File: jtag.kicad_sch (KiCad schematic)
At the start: 49 parts, among them J3 USB_C_Receptacle, J4 Conn_01x02_Male, J5 3220-10-0100-00, U2 FT2232HL-REEL, U3 74LVC1G125, U4 74LVC1G125, U5 74LVC1G125, U6 74LVC1G125, U7 74LVC1G125, Y2 12MHz

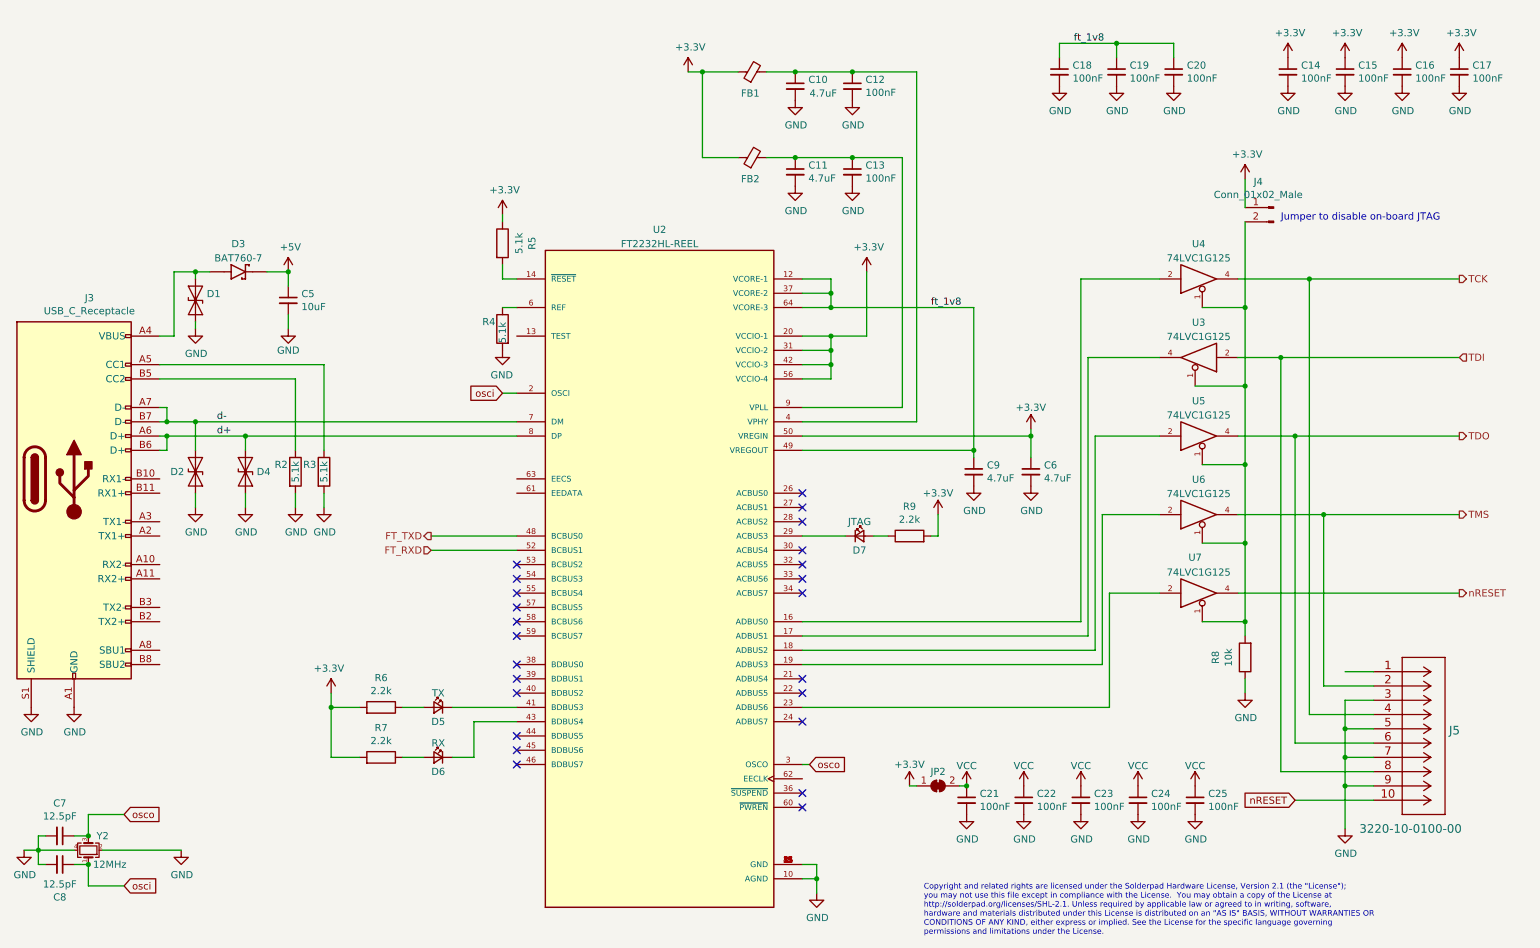
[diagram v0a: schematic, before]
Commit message: Power and Level Shifter updates
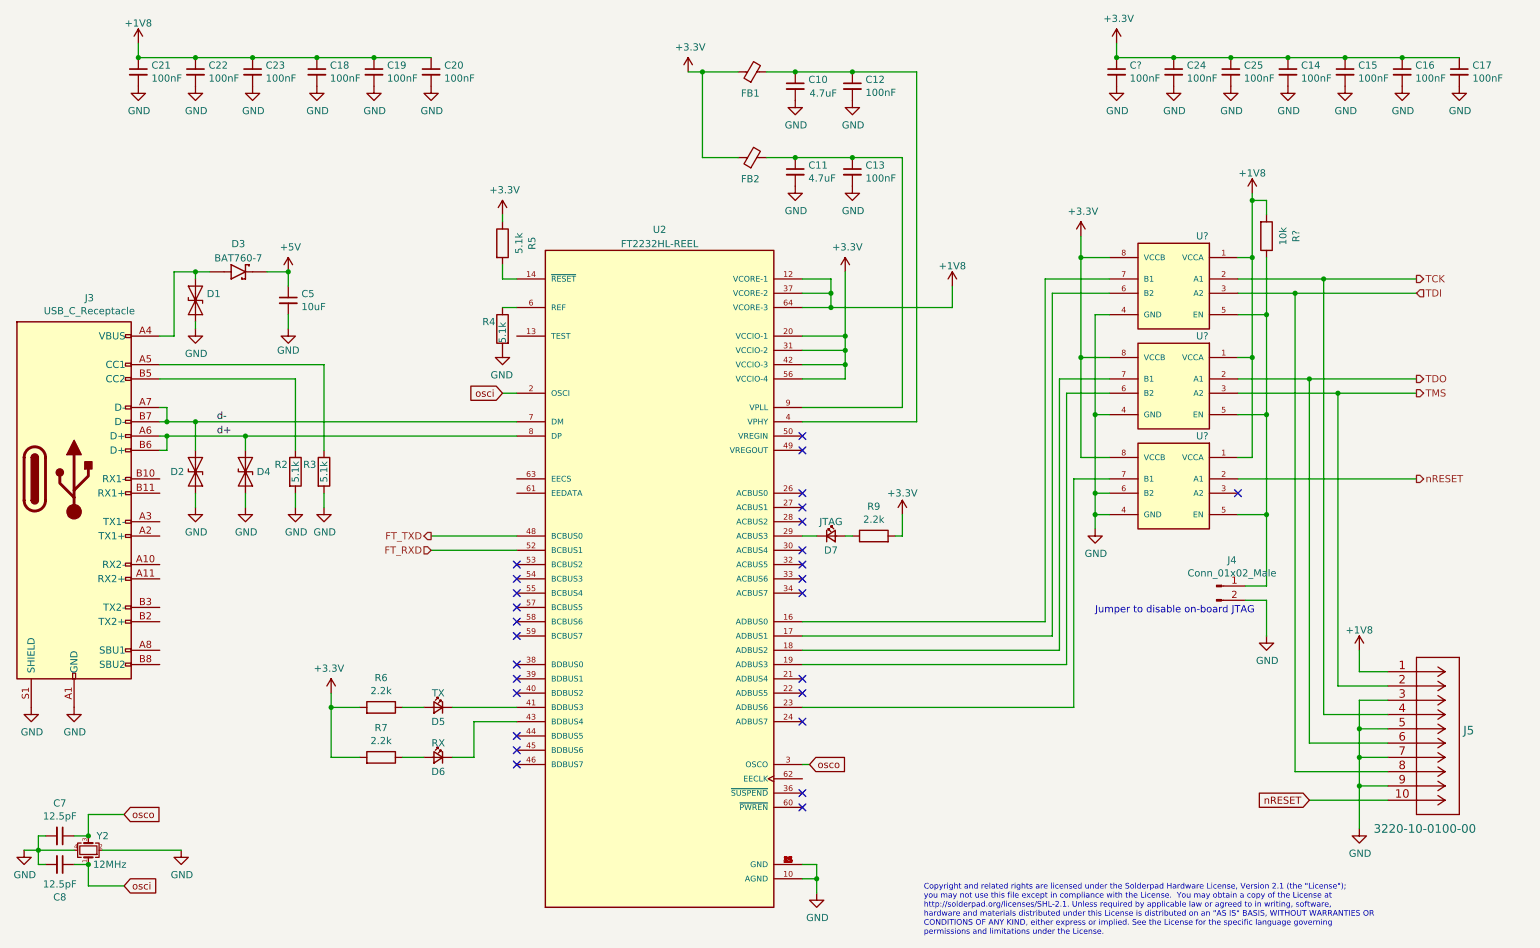
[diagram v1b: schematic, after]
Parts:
- removed C6, C9: 4.7uF, Capacitor_SMD:C_0603_1608Metric_Pad1.08x0.95mm_HandSolder, symbol Device:C_Small
- removed JP2: SolderJumper_2_Bridged, Jumper:SolderJumper-2_P1.3mm_Bridged_RoundedPad1.0x1.5mm, symbol Jumper:SolderJumper_2_Bridged
- removed R8: 10k, Resistor_SMD:R_0603_1608Metric_Pad0.98x0.95mm_HandSolder, symbol Device:R
- removed U3, U4, U5, U6, U7: 74LVC1G125, Package_TO_SOT_SMD:SOT-353_SC-70-5, symbol 74xGxx:74LVC1G125
- added C?: 100nF, Capacitor_SMD:C_0603_1608Metric_Pad1.08x0.95mm_HandSolder, symbol Device:C_Small
- added R?: 10k, Resistor_SMD:R_0603_1608Metric_Pad0.98x0.95mm_HandSolder, symbol Device:R
- added U? (x3): PI4ULS3V302XVEX, PSON40P160X120X55-8N, symbol PI4ULS3V302XVEX:PI4ULS3V302XVEX
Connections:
- net +3V3: now also C24.1, C25.1, C?.1, U?.8 (VCCB), U?.8 (VCCB), U?.8 (VCCB); no longer J4.1 (Pin_1), U2.50 (VREGIN)
- net GND: now also J4.2 (Pin_2), C?.2, U?.4 (GND), U?.4 (GND), U?.4 (GND), U?.6 (B2)
- net TCK: now also U?.2 (A1)
- net TDI: now also U?.3 (A2)
- net TDO: now also U?.2 (A1)
- net TMS: now also U?.3 (A2)
- net nRESET: now also U?.2 (A1)
- net at U2.19 (ADBUS3): now also U?.6 (B2)
- net at U2.23 (ADBUS6): now also U?.7 (B1)
- net at U2.18 (ADBUS2): now also U?.7 (B1)
- net +1V8: now reaches J5.1
- net +1V8: now also C18.1, C19.1, C20.1, C21.1, C22.1, C23.1, U2.12 (VCORE-1), U2.37 (VCORE-2), U2.64 (VCORE-3), R?.2, U?.1 (VCCA), U?.1 (VCCA), U?.1 (VCCA)
- net at U2.16 (ADBUS0): now also U?.7 (B1)
- net at U2.17 (ADBUS1): now also U?.6 (B2)
- removed net VCC: C21.1, C22.1, C23.1, C24.1, C25.1
- removed net ft_1v8: C18.1, C19.1, C20.1, U2.12 (VCORE-1), U2.37 (VCORE-2), U2.49 (VREGOUT), U2.64 (VCORE-3)
- new net: J4.1 (Pin_1), R?.1, U?.5 (EN), U?.5 (EN), U?.5 (EN)
- no-connect marks 24 -> 27
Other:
- moved on the sheet: C18, C19, C20, C21, C22, C23, C24, C25, D7, J4, J5, R9
